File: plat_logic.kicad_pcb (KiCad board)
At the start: 2 copper layers, 100 x 100 mm, 133 parts, among them CN1 GPS_Port, Con2 DS1023-1X2SF11, J1 USB_C_Receptacle, J10 DS1023-1X8SF11, J11 DS1023-1X5SF11, J12 DS1023-1X5SF11, J13 DS1023-1X5SF11, J14 DS1023-1X5SF11, J15 DS1023-1X5SF11, J16 DS1023-1X5SF11, J17 DS1023-1X5SF11, J2 JST_GH_SM06B-GHS-TB, J3 JST_GH_SM06B-GHS-TB, J4 JST_GH_SM06B-GHS-TB, J5 JST_GH_SM06B-GHS-TB, J6 DS1023-1X11S21, J7 DS1023-1X11S21, J8 DS1023-1X6SF11, J9 DS1023-1X11S21, SW1 Button-SMD-4.5x4.5x5.5, SW2 Button-SMD-4.5x4.5x5.5, U1 STM32F429ZITx, U2 USBLC6-2SC6, U3 SN65HVD232, Y2 NX3215SA-32.768KHZ-EXS00A-MU0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, Y3 CSTNE8M00GH5L000R0 8.000MHZ, con1 DS1023-1X3SF11

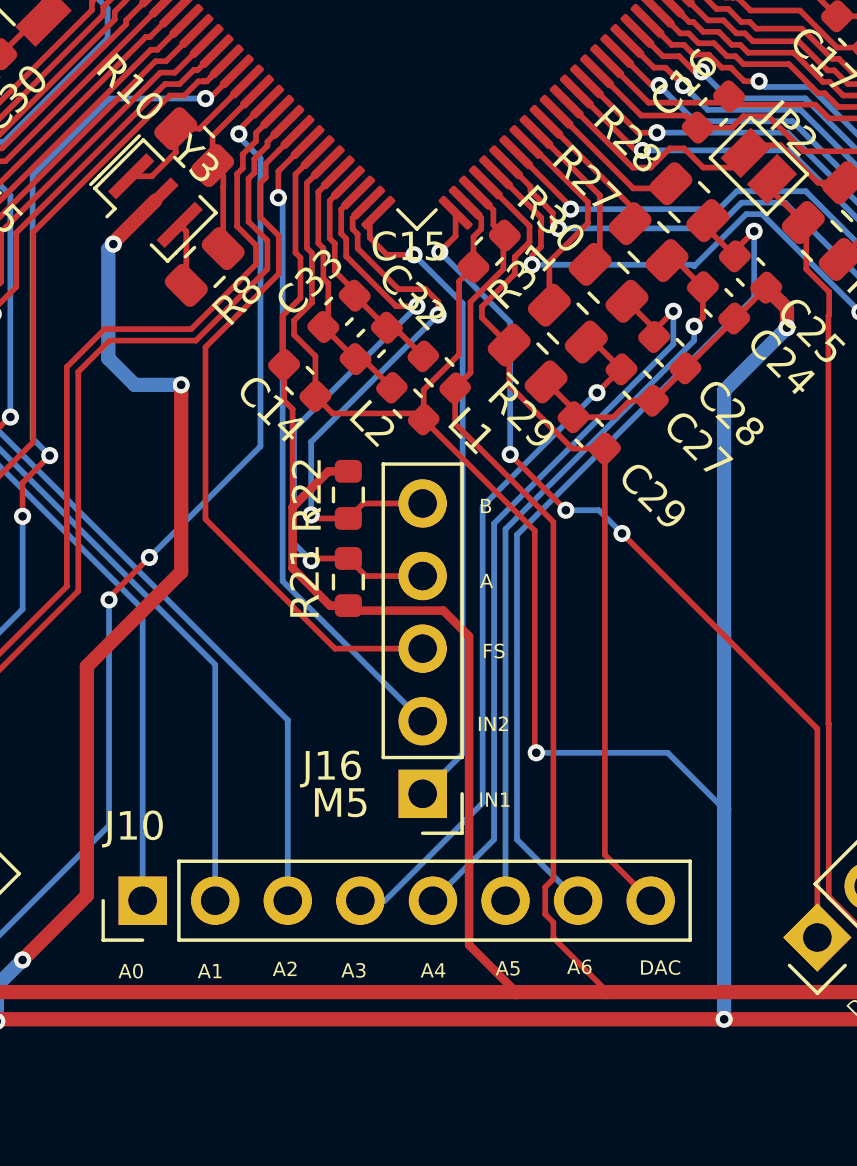
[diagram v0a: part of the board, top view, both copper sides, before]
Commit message: Финал
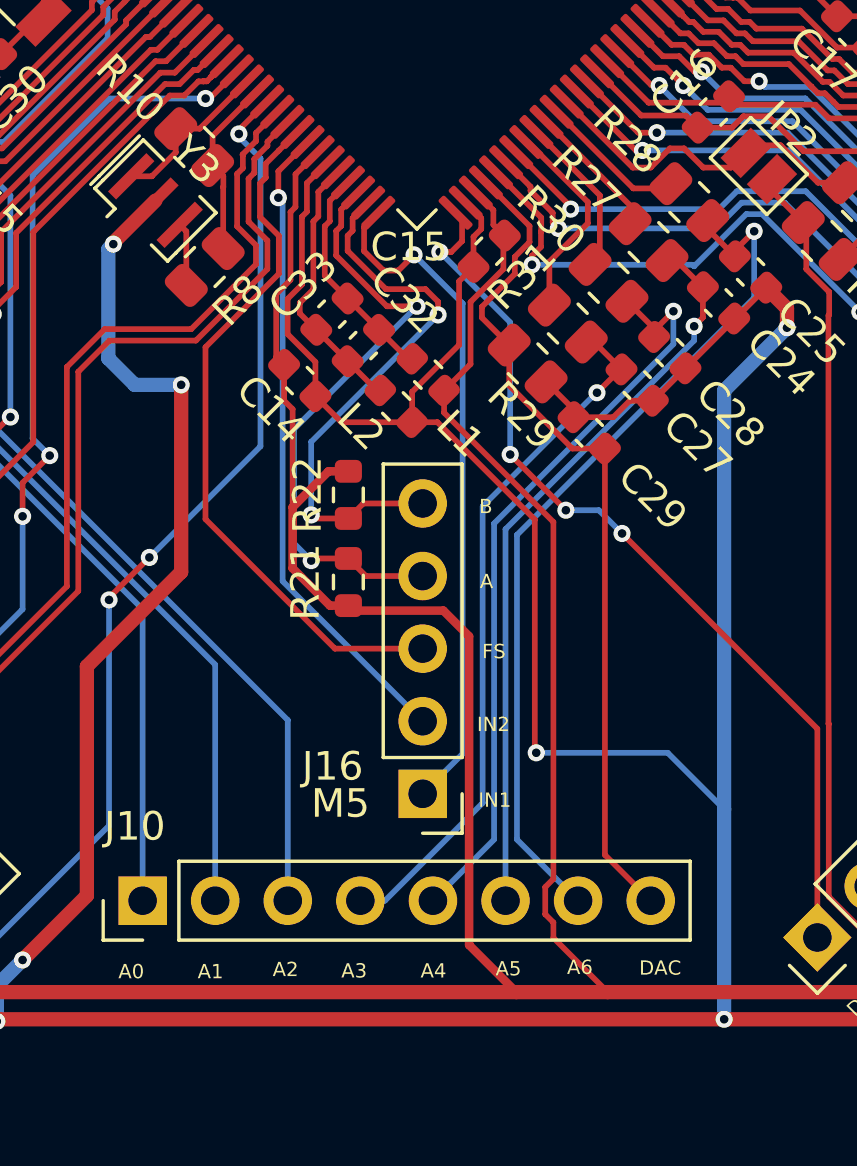
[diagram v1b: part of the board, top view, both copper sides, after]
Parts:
- moved L2 0.41 mm to (150.1, 122.5)
- moved L1 0.40 mm to (151.2, 121.4)
- moved C32 0.29 mm to (148.9, 120.4)
- moved C33 0.27 mm to (147.8, 119.3)
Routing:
- net IN1_M5: track 22.9 -> 24.0 mm
- net GND: track 905.5 -> 906.3 mm
